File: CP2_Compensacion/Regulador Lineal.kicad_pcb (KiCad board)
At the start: 2 copper layers, 64 x 51 mm, 24 parts, among them J1 conn_vreg, J2 conn_vreg, J3 conn_rl_gnd, J4 conn_rl, Q1 BD140, Q10 BD139, Q2 BD140, Q3 BD139, Q4 BD139, Q5 TIP42C, Q6 BD139, Q7 BD139, Q8 BD139, U1 TL431LP

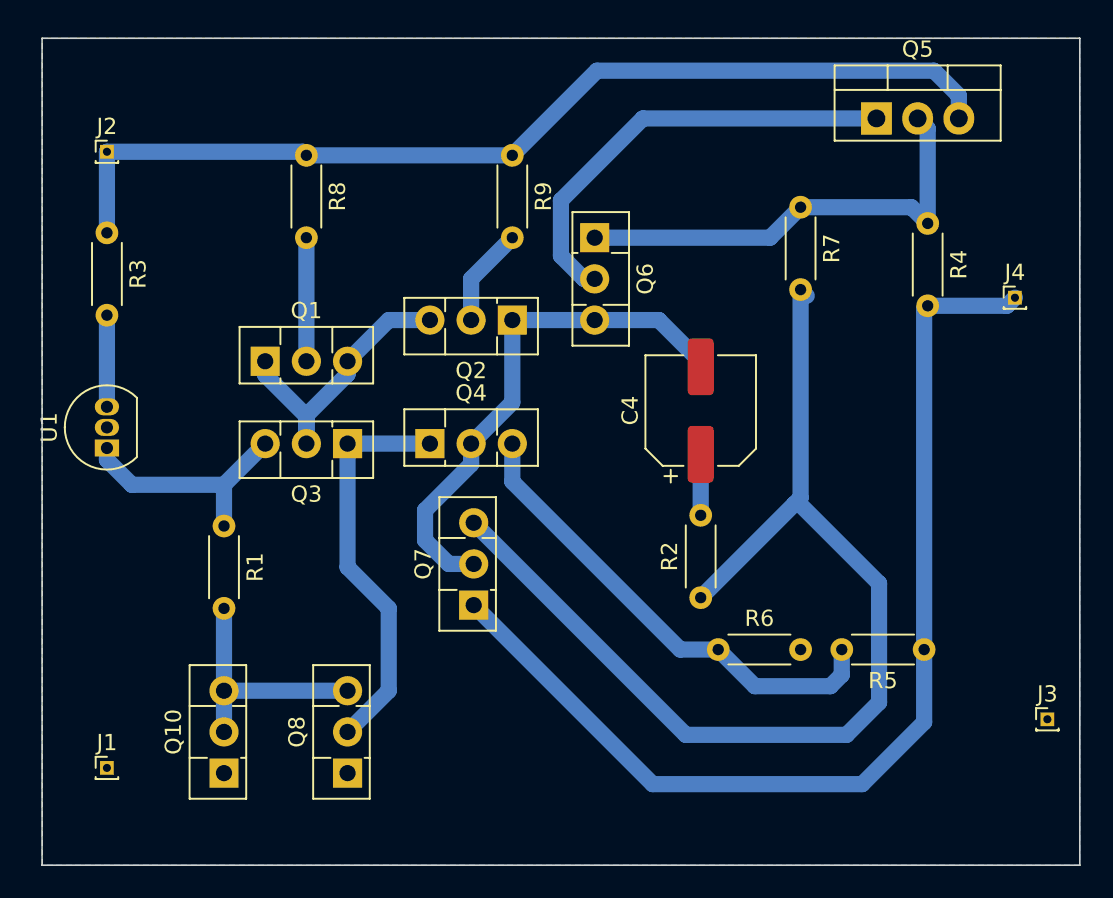
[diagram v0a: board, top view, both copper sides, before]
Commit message: Add files via upload
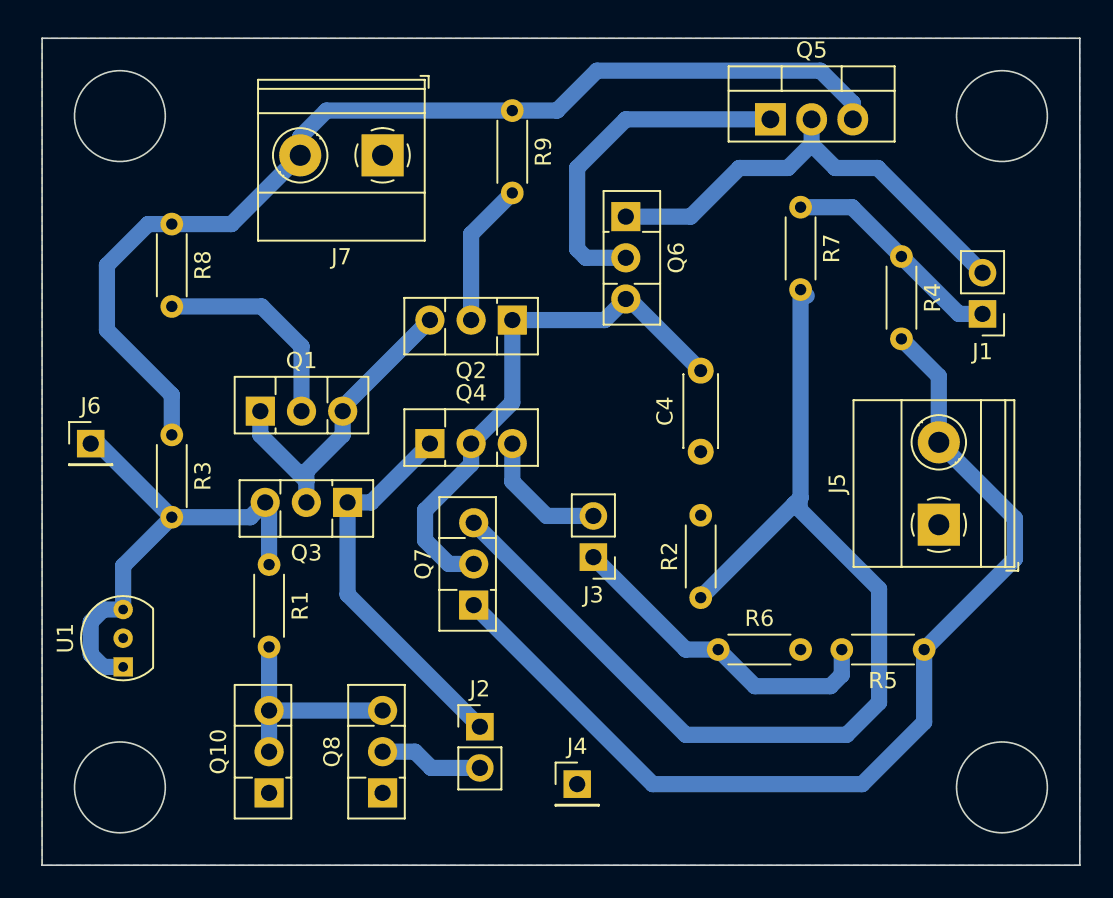
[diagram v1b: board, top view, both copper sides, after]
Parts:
- added J5: out, TerminalBlock_Phoenix:TerminalBlock_Phoenix_MKDS-1,5-2-5.08_1x02_P5.08mm_Horizontal, F.Cu at (166.3, 73.0)
- added J6: V1, Connector_PinHeader_2.54mm:PinHeader_1x01_P2.54mm_Vertical, F.Cu at (114.0, 68.0)
- added J7: in, TerminalBlock_Phoenix:TerminalBlock_Phoenix_MKDS-1,5-2-5.08_1x02_P5.08mm_Horizontal, F.Cu at (132.0, 50.2)
- C4: footprint Capacitor_SMD:CP_Elec_6.3x4.5 -> Capacitor_THT:C_Disc_D4.3mm_W1.9mm_P5.00mm
- J1: value conn_vreg -> I1; footprint Connector_PinHeader_1.00mm:PinHeader_1x01_P1.00mm_Vertical -> Connector_PinHeader_2.54mm:PinHeader_1x02_P2.54mm_Vertical
- J2: value conn_vreg -> I2; footprint Connector_PinHeader_1.00mm:PinHeader_1x01_P1.00mm_Vertical -> Connector_PinHeader_2.54mm:PinHeader_1x02_P2.54mm_Vertical
- J3: value conn_rl_gnd -> I3; footprint Connector_PinHeader_1.00mm:PinHeader_1x01_P1.00mm_Vertical -> Connector_PinHeader_2.54mm:PinHeader_1x02_P2.54mm_Vertical
- J4: value conn_rl -> gnd; footprint Connector_PinHeader_1.00mm:PinHeader_1x01_P1.00mm_Vertical -> Connector_PinHeader_2.54mm:PinHeader_1x01_P2.54mm_Vertical
- moved J1 60.8 mm to (169.0, 60.0), turned to 180 degrees
- moved J2 42.3 mm to (138.0, 85.5)
- moved J4 40.4 mm to (144.0, 89.0)
- moved J3 29.7 mm to (145.0, 75.0), turned to 180 degrees
- moved R3 13.1 mm to (119.0, 67.5)
- moved U1 13.0 mm to (116.0, 81.3)
- moved R8 9.32 mm to (119.0, 54.5)
- moved Q5 6.54 mm to (155.9, 48.0)
- moved R1 3.66 mm to (125.0, 75.5)
- moved Q3 3.62 mm to (129.8, 71.6)
- moved Q1 3.09 mm to (124.5, 66.0)
- moved Q10 3.04 mm to (125.0, 89.5)
- moved R9 2.76 mm to (140.0, 47.5)
- moved R4 2.60 mm to (164.0, 56.5)
- moved C4 2.54 mm to (151.6, 68.5)
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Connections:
- J1 pad 1: GND -> Net-(J1-Pin_1)
- J3 pad 1: GND -> Net-(J3-Pin_1)
- J4 pad 1: Net-(J4-Pin_1) -> GND
- Q3 pad 1: Net-(Q3-E) -> Net-(J2-Pin_1)
- Q4 pad 1: Net-(Q3-E) -> Net-(J2-Pin_1)
- Q4 pad 3: Net-(Q4-B) -> Net-(J3-Pin_2)
- Q5 pad 2: Net-(Q5-C) -> Net-(J1-Pin_2)
- Q5 pad 3: Net-(J2-Pin_1) -> Net-(J7-Pin_2)
- Q6 pad 1: Net-(Q5-C) -> Net-(J1-Pin_2)
- Q7 pad 1: Net-(J4-Pin_1) -> Net-(J5-Pin_2)
- Q8 pad 2: Net-(Q3-E) -> Net-(J2-Pin_2)
- R3 pad 1: Net-(J2-Pin_1) -> Net-(J7-Pin_2)
- R4 pad 1: Net-(Q5-C) -> Net-(J1-Pin_1)
- R4 pad 2: Net-(J4-Pin_1) -> Net-(J5-Pin_2)
- R5 pad 1: Net-(J4-Pin_1) -> Net-(J5-Pin_2)
- R5 pad 2: Net-(Q4-B) -> Net-(J3-Pin_1)
- R6 pad 1: Net-(Q4-B) -> Net-(J3-Pin_1)
- R7 pad 1: Net-(Q5-C) -> Net-(J1-Pin_1)
- R8 pad 1: Net-(J2-Pin_1) -> Net-(J7-Pin_2)
- R9 pad 1: Net-(J2-Pin_1) -> Net-(J7-Pin_2)
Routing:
- net Net-(J7-Pin_2): track 0.00 -> 65.6 mm
- net Net-(J4-Pin_1): track 65.3 -> 0.00 mm
- net Net-(J5-Pin_2): track 0.00 -> 62.8 mm
- net Net-(J2-Pin_1): track 61.8 -> 23.8 mm
- net Net-(Q4-B): track 29.7 -> 0.00 mm
- net Net-(J1-Pin_2): track 0.00 -> 28.7 mm
- net Net-(Q5-C): track 28.5 -> 0.00 mm
- net Net-(Q3-E): track 25.0 -> 0.00 mm
- net Net-(J3-Pin_1): track 0.00 -> 20.5 mm
- net Net-(J1-Pin_1): track 0.00 -> 13.9 mm
- net Net-(J6-Pin_1): track 20.4 -> 30.5 mm
- net Net-(J3-Pin_2): track 0.00 -> 8.22 mm
- net Net-(J2-Pin_2): track 0.00 -> 6.41 mm
- net Net-(Q5-B): track 27.6 -> 21.4 mm
- net Net-(Q1-C): track 7.62 -> 13.0 mm
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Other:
- outline, holes or cut-outs redrawn
